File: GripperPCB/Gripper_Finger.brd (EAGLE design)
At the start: 26.6 x 50.5 mm, 10 parts, among them IC1 ATMEGA328PB-AU, IC2 L293D, IC3 L293D

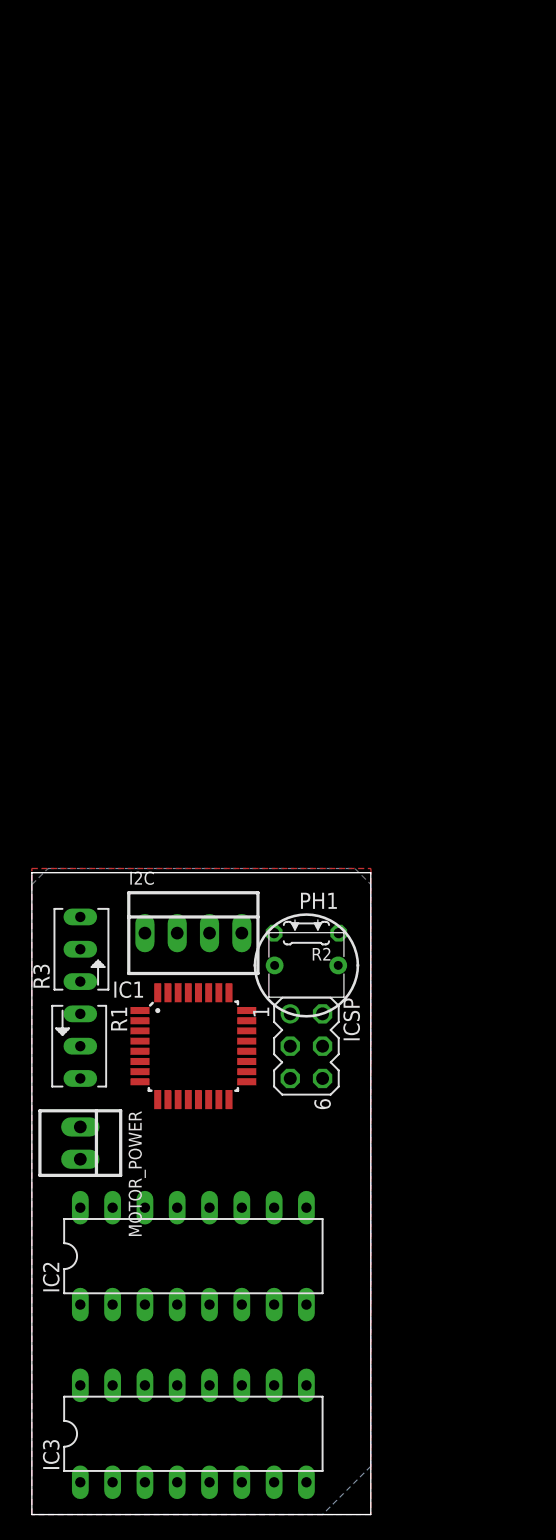
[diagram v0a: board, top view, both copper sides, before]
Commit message: version 1.0.0 sent to engineering
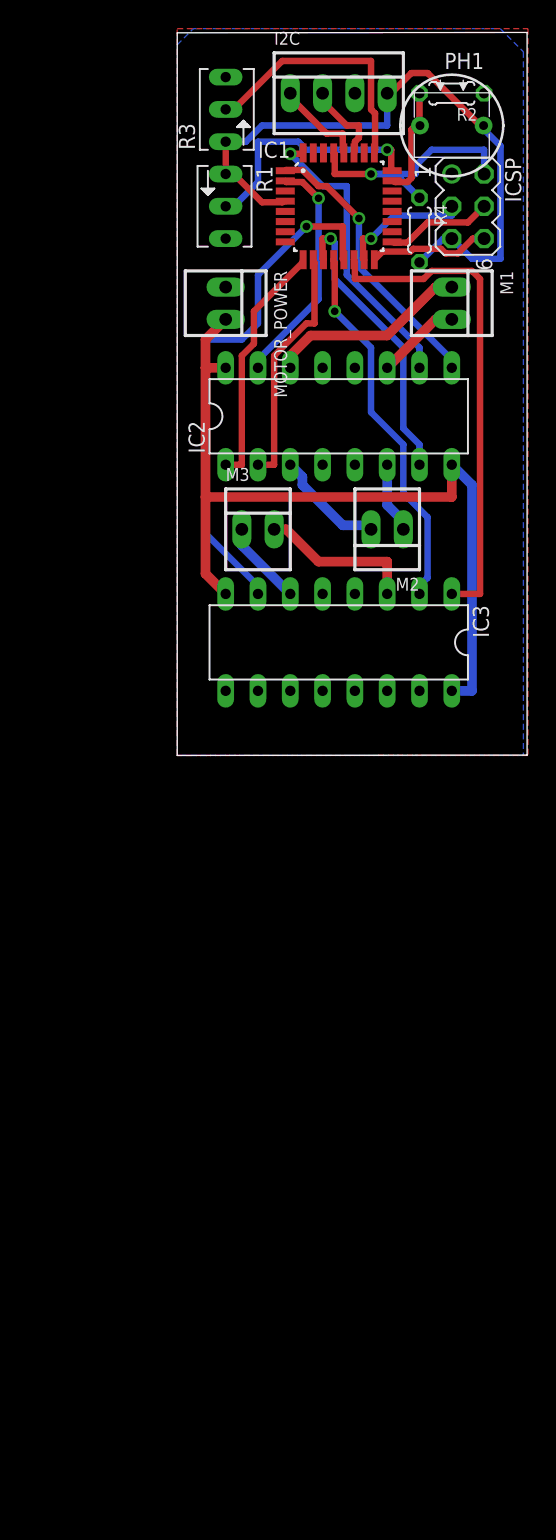
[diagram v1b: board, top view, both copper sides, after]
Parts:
- added M1, M2, M3: 22-23-2021, con-molex:22-23-2021
- added R4: (no value), rcl:0204/5
- moved ICSP 67.3 mm to (34.3, 72.4)
- moved I2C 67.0 mm to (24.1, 81.3)
- moved IC1 67.0 mm to (24.1, 72.4)
- moved IC2 67.0 mm to (24.1, 55.9)
- moved R1 67.0 mm to (15.2, 72.4)
- moved R2 67.0 mm to (33.0, 81.3)
- moved R3 67.0 mm to (15.2, 80.0)
- moved MOTOR_POWER 67.0 mm to (15.2, 64.8)
- moved PH1 67.0 mm to (33.0, 78.7)
- moved IC3 63.3 mm to (24.1, 38.1), turned to 180 degrees
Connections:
- net N$1 renamed SCL
- net N$10 renamed MOTOR_POWER
- net N$2 renamed SDA
- net N$4 renamed SCK
- net N$5 renamed MISO
- net N$6 renamed MOSI
- net N$7 renamed LIGHT
- net N$8 renamed POT1
- net N$9 renamed POT2
- removed net N$3: IC1.29, ICSP.2
- new net M1A: IC2.14, M1.1
- new net M1B: IC2.11, M1.2
- new net M2A: IC2.3, M2.2
- new net M2B: IC2.6, M2.1
- new net M3A: IC3.6, M3.1
- new net M3B: IC3.3, M3.2
- new net N$11: IC1.32, IC2.10
- new net N$12: IC1.1, IC2.9
- new net N$13: IC1.2, IC2.15
- new net N$20: IC1.9, IC2.1
- new net N$21: IC1.10, IC2.2
- new net N$22: IC1.11, IC2.7
- new net N$23: IC1.13, IC3.7
- new net N$24: IC1.12, IC3.2
- new net N$25: IC1.14, IC3.1
- new net RESET: IC1.29, ICSP.2, R4.1
- net VCC: now also R4.2
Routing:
- net MOTOR_POWER: track 0.00 -> 66.4 mm
- net VCC: track 0.00 -> 52.7 mm
- net N$23: track 0.00 -> 41.1 mm, vias 0 -> 1
- net N$25: track 0.00 -> 38.9 mm
- net N$24: track 0.00 -> 29.6 mm, vias 0 -> 1
- net N$11: track 0.00 -> 23.2 mm, vias 0 -> 1
- net N$22: track 0.00 -> 23.0 mm, vias 0 -> 1
- net N$12: track 0.00 -> 22.2 mm, vias 0 -> 1
- net RESET: track 0.00 -> 21.1 mm, vias 0 -> 1
- net POT2: track 0.00 -> 20.4 mm
- net N$20: track 0.00 -> 19.4 mm
- net POT1: track 0.00 -> 19.1 mm, vias 0 -> 1
- net N$21: track 0.00 -> 19.1 mm
- net N$13: track 0.00 -> 18.5 mm, vias 0 -> 1
- net M1A: track 0.00 -> 15.9 mm
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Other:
- board size 26.6 x 50.5 mm -> 27.5 x 56.9 mm
